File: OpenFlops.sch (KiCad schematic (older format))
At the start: 82 parts, among them J99 OSHW_LOGO, P1 FLOPPY_CONN, P2 POWER_INPUT, P3 USB_A_FEMALE, P4 PROG_PORT, P5 JUMPERS, P6 ENCODER_PORT, P7 DISPLAY_PORT, P8 USB_HEADER, P9 EXTERNAL_SPEAKER, Q1 MOS_N_GSD, Q2 MOS_N_GSD, Q3 MOS_N_GSD, Q4 MOS_N_GSD, Q5 MOS_N_GSD, Q6 MOS_N_GSD, Q7 MMBT3904, U1 74HCT04, U3 STM32F105RBT6, U4 LM1117-3.3, Y1 8 MHz

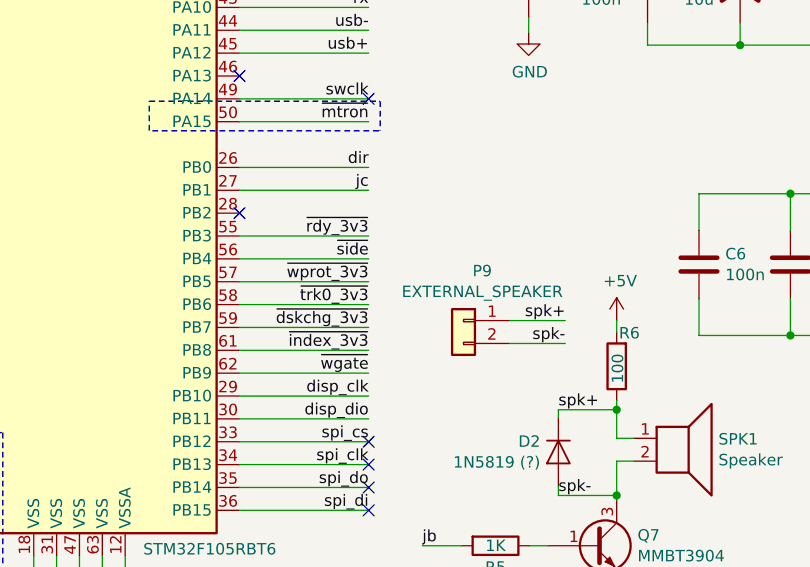
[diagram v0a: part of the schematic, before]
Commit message: Fix #4
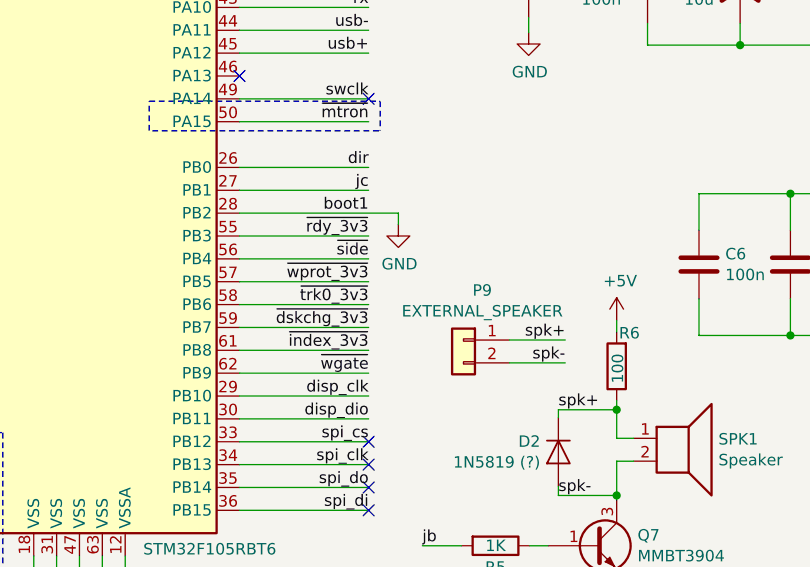
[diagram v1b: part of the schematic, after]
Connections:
- net GND: now also U3.28 (PB2)
- no-connect marks 22 -> 21
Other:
- moved on the sheet: P9
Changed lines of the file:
@@
 NoConn ~ 3255 1900
 NoConn ~ 3255 2600
-NoConn ~ 3255 3200
 NoConn ~ 1855 2800
 NoConn ~ 1855 3900
@@
 L Connector_Generic:Conn_01x02 P9
 U 1 1 5D86073A
-P 4235 3670
-F 0 "P9" H 4153 3887 50  0000 C CNN
-F 1 "EXTERNAL_SPEAKER" H 4153 3796 50  0000 C CNN
-F 2 "OpenFlops:PinHeader_1x02_P2.54mm_Mute" H 4235 3670 50  0001 C CNN
-F 3 "~" H 4235 3670 50  0001 C CNN
-	1    4235 3670
+P 4235 3755
+F 0 "P9" H 4153 3972 50  0000 C CNN
+F 1 "EXTERNAL_SPEAKER" H 4153 3881 50  0000 C CNN
+F 2 "OpenFlops:PinHeader_1x02_P2.54mm_Mute" H 4235 3755 50  0001 C CNN
+F 3 "~" H 4235 3755 50  0001 C CNN
+	1    4235 3755
 	-1   0    0    -1
 $EndComp
 Wire Wire Line
-	4435 3670 4680 3670
-Wire Wire Line
-	4435 3770 4680 3770
+	4435 3755 4680 3755
+Wire Wire Line
+	4435 3855 4680 3855
 Wire Wire Line
 	4650 4435 4650 4395
@@
 Text Label 4650 4435 0    50   ~ 0
 spk-
-Text Label 4680 3770 2    50   ~ 0
+Text Label 4680 3855 2    50   ~ 0
 spk-
 Text Label 4650 4060 0    50   ~ 0
 spk+
-Text Label 4680 3670 2    50   ~ 0
+Text Label 4680 3755 2    50   ~ 0
 spk+
 Text Label 7495 1050 0    50   ~ 0
@@
 	0    1    1    0
 $EndComp
+Text Label 3820 3200 2    50   ~ 0
+boot1
+$Comp
+L power:GND #PWR?
+U 1 1 5E2952AE
+P 3950 3250
+F 0 "#PWR?" H 3950 3000 50  0001 C CNN
+F 1 "GND" H 3955 3077 50  0000 C CNN
+F 2 "" H 3950 3250 50  0001 C CNN
+F 3 "" H 3950 3250 50  0001 C CNN
+	1    3950 3250
+	1    0    0    -1
+$EndComp
+Wire Wire Line
+	3950 3200 3950 3250
+Wire Wire Line
+	3255 3200 3950 3200
 $EndSCHEMATC
